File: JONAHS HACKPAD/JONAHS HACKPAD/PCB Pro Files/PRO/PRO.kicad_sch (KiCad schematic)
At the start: 42 parts, among them SW2 SW_Push, SW3 SW_Push, SW4 SW_Push, SW5 SW_Push, U1 MOUDLE-SEEEDUINO-XIAO, U2 OLED_0.91_128x32

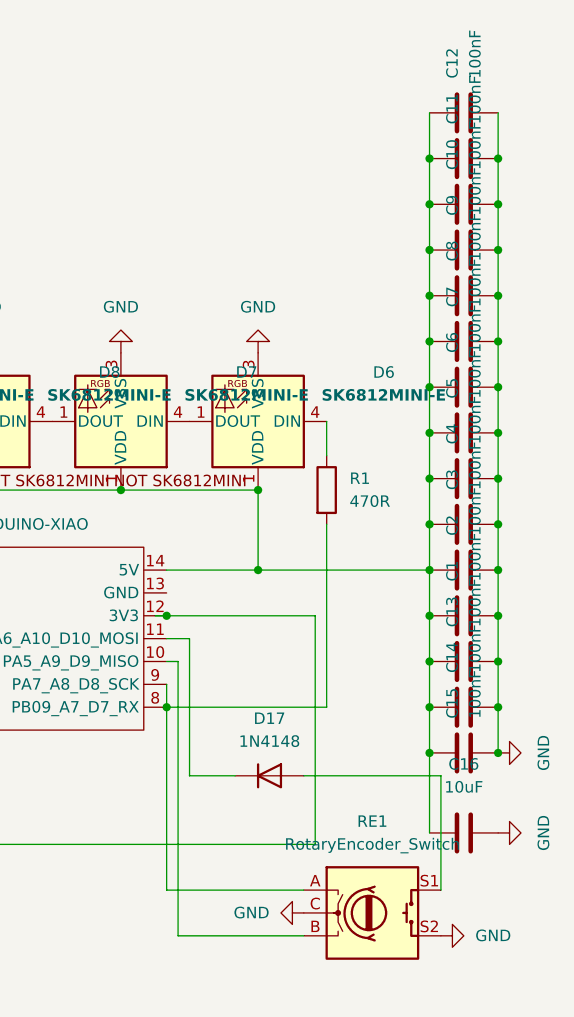
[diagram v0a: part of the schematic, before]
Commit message: update stuff
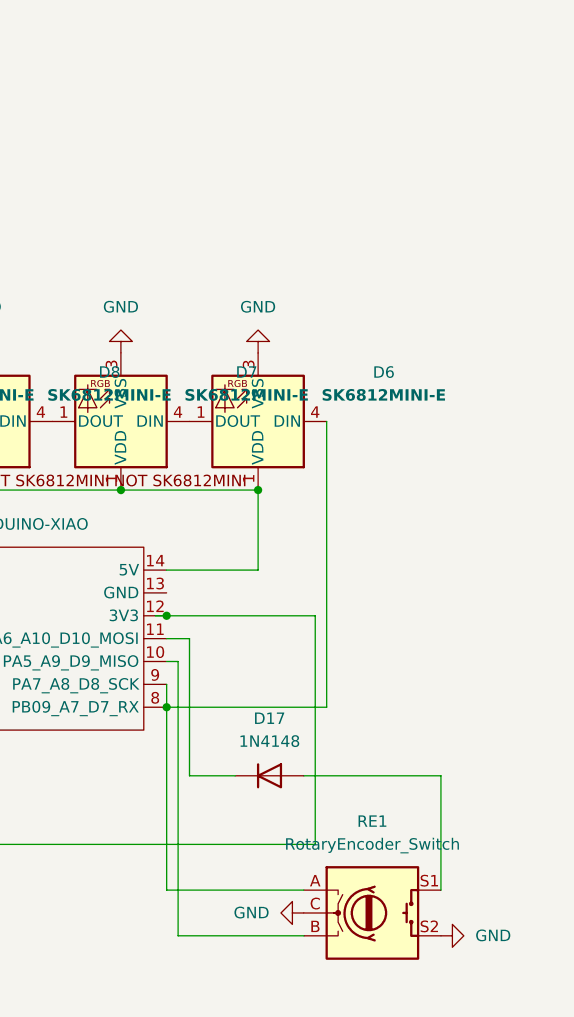
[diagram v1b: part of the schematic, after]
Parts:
- removed C1, C10, C11, C12, C13, C14, C15, C2, C3, C4, C5, C6, C7, C8, C9: 100nF, Capacitor_SMD:C_0805_2012Metric, symbol Device:C
- removed C16: 10uF, Capacitor_SMD:C_0805_2012Metric, symbol Device:C
- removed R1: 470R, Resistor_SMD:R_0805_2012Metric, symbol Device:R
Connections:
- net at D10.1 (DOUT): now also D11.1 (DOUT), D12.1 (DOUT), D13.1 (DOUT), D14.1 (DOUT), D15.1 (DOUT), D16.1 (DOUT), D6.1 (DOUT), D7.1 (DOUT), D8.1 (DOUT), D9.1 (DOUT), U1.14 (5V)
- net at RE1.A, U1.8 (PB09_A7_D7_RX), U1.9 (PA7_A8_D8_SCK): now also D6.4 (DIN)
- now unconnected: D16.1 (DOUT)
